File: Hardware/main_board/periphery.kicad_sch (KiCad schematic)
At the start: 67 parts, among them J4 SD, J5 NFC, J6 EXT1, J7 EXT0, U12 LP5562TMX

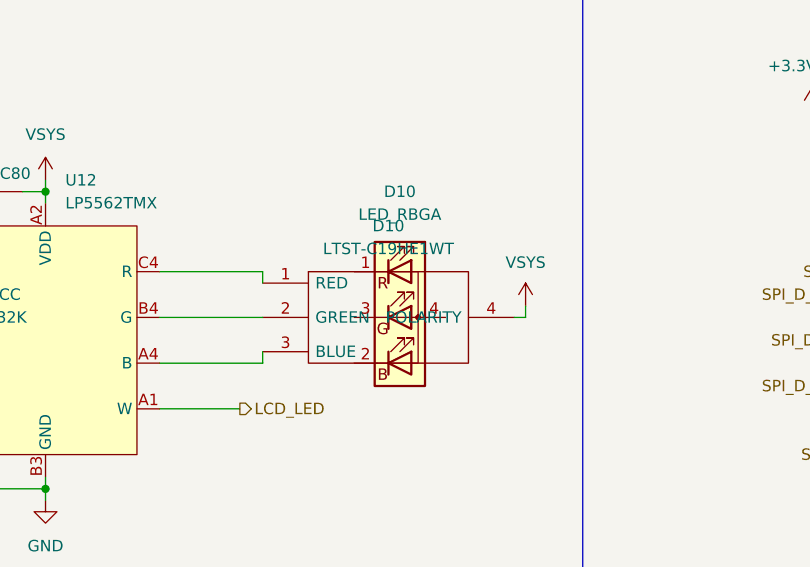
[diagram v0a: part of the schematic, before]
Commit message: misc: fix conflict
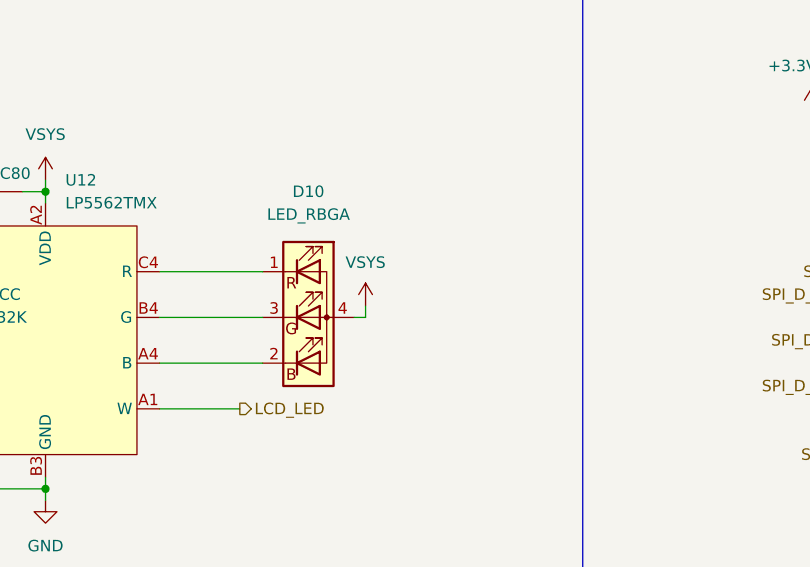
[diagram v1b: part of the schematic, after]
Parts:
- removed D10: LTST-C19HE1WT, Library:LTST-C19HE1WT, symbol Library:LTST-C19HE1WT
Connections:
- net VSYS: now also D10.4 (A)
- net at U12.C4 (R): now also D10.1 (RK)
- net at U12.B4 (G): now also D10.3 (GK)
- net at U12.A4 (B): now also D10.2 (BK)
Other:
- moved on the sheet: D10
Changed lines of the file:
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@@
 	(wire
 		(pts
-			(xy 74.93 44.45) (xy 74.93 45.72)
-		)
-		(stroke
-			(width 0)
-			(type default)
-		)
-	)
-	(wire
-		(pts
 			(xy 234.95 139.7) (xy 223.52 139.7)
 		)
@@
 	(wire
 		(pts
-			(xy 102.87 49.53) (xy 104.14 49.53)
+			(xy 85.09 49.53) (xy 86.36 49.53)
 		)
 		(stroke
@@
 	(wire
 		(pts
-			(xy 74.93 54.61) (xy 74.93 53.34)
-		)
-		(stroke
-			(width 0)
-			(type default)
-		)
-	)
-	(wire
-		(pts
 			(xy 78.74 144.78) (xy 85.09 144.78)
 		)
@@
 	(wire
 		(pts
-			(xy 104.14 49.53) (xy 104.14 48.26)
+			(xy 86.36 49.53) (xy 86.36 48.26)
 		)
 		(stroke
@@
 	)
 	(symbol
-		(lib_id "Library:LTST-C19HE1WT")
-		(at 74.93 45.72 0)
-		(unit 1)
-		(exclude_from_sim no)
-		(in_bom yes)
-		(on_board yes)
-		(dnp no)
-		(fields_autoplaced yes)
-		(property "Reference" "D10"
-			(at 88.9 39.37 0)
-			(effects
-				(font
-					(size 1.27 1.27)
-				)
-			)
-		)
-		(property "Value" "LTST-C19HE1WT"
-			(at 88.9 41.91 0)
-			(effects
-				(font
-					(size 1.27 1.27)
-				)
-			)
-		)
-		(property "Footprint" "Library:LTST-C19HE1WT"
-			(at 130.556 37.338 0)
-			(effects
-				(font
-					(size 1.27 1.27)
-				)
-				(justify left)
-				(hide yes)
-			)
-		)
-		(property "Datasheet" "https://datasheet.datasheetarchive.com/originals/distributors/Datasheets-DGA13/1159767.pdf"
-			(at 130.556 39.878 0)
-			(effects
-				(font
-					(size 1.27 1.27)
-				)
-				(justify left)
-				(hide yes)
-			)
-		)
-		(property "Description" "LED,SMD,1.6x1.5x0.4mm,Red/Green/Blue Lite-On LTST-C19HE1WT 3 RGB LED, 470 / 525 / 624 nm 3-Pin, Rectangle Lens SMD package"
-			(at 130.556 42.418 0)
-			(effects
-				(font
-					(size 1.27 1.27)
-				)
-				(justify left)
-				(hide yes)
-			)
-		)
-		(property "Height" ""
-			(at 106.68 50.8 0)
-			(effects
-				(font
-					(size 1.27 1.27)
-				)
-				(justify left)
-				(hide yes)
-			)
-		)
-		(property "Mouser Part Number" "859-LTST-C19HE1WT"
-			(at 130.556 47.498 0)
-			(effects
-				(font
-					(size 1.27 1.27)
-				)
-				(justify left)
-				(hide yes)
-			)
-		)
-		(property "Mouser Price/Stock" "https://www.mouser.co.uk/ProductDetail/Lite-On/LTST-C19HE1WT?qs=WAWaI72GHKxJLPArJA9%252BUw%3D%3D"
-			(at 130.556 50.038 0)
-			(effects
-				(font
-					(size 1.27 1.27)
-				)
-				(justify left)
-				(hide yes)
-			)
-		)
-		(property "Manufacturer_Name" "Lite-On"
-			(at 130.556 52.578 0)
-			(effects
-				(font
-					(size 1.27 1.27)
-				)
-				(justify left)
-				(hide yes)
-			)
-		)
-		(property "Manufacturer_Part_Number" "LTST-C19HE1WT"
-			(at 130.556 55.118 0)
-			(effects
-				(font
-					(size 1.27 1.27)
-				)
-				(justify left)
-				(hide yes)
-			)
-		)
-		(pin "3"
-		)
-		(pin "4"
-		)
-		(pin "2"
-		)
-		(pin "1"
-		)
-		(instances
-			(project "main_board"
-				(path "/16216a68-6dea-41d7-8e15-2cc84f72f8e2/07054158-43be-4dab-a684-c4a4bca9b970"
-					(reference "D10")
-					(unit 1)
-				)
-			)
-		)
-	)
-	(symbol
 		(lib_id "Device:R_US")
 		(at 147.32 35.56 180)
@@
 	(symbol
 		(lib_id "Device:LED_RBGA")
-		(at 90.17 49.53 0)
+		(at 80.01 49.53 0)
 		(unit 1)
 		(exclude_from_sim no)
@@
 		(fields_autoplaced yes)
 		(property "Reference" "D10"
-			(at 90.17 35.56 0)
+			(at 80.01 35.56 0)
 			(effects
 				(font
@@
 		)
 		(property "Value" "LED_RBGA"
-			(at 90.17 38.1 0)
+			(at 80.01 38.1 0)
 			(effects
 				(font
@@
 		)
 		(property "Footprint" "Library:LTST-C19HE1WT_LTO"
-			(at 90.17 50.8 0)
+			(at 80.01 50.8 0)
 			(effects
 				(font
@@
 		)
 		(property "Datasheet" "~"
-			(at 90.17 50.8 0)
+			(at 80.01 50.8 0)
 			(effects
 				(font
@@
 		)
 		(property "Description" "RGB LED, red/blue/green/anode"
-			(at 90.17 49.53 0)
+			(at 80.01 49.53 0)
 			(effects
 				(font
@@
 	(symbol
 		(lib_id "power:+3.3V")
-		(at 104.14 48.26 0)
+		(at 86.36 48.26 0)
 		(unit 1)
 		(exclude_from_sim no)
@@
 		(dnp no)
 		(property "Reference" "#PWR0122"
-			(at 104.14 52.07 0)
+			(at 86.36 52.07 0)
 			(effects
 				(font
@@
 		)
 		(property "Value" "VSYS"
-			(at 104.14 43.434 0)
+			(at 86.36 43.434 0)
 			(effects
 				(font
@@
 		)
 		(property "Footprint" ""
-			(at 104.14 48.26 0)
+			(at 86.36 48.26 0)
 			(effects
 				(font
@@
 		)
 		(property "Datasheet" ""
-			(at 104.14 48.26 0)
+			(at 86.36 48.26 0)
 			(effects
 				(font
@@
 		)
 		(property "Description" "Power symbol creates a global label with name \"+3.3V\""
-			(at 104.14 48.26 0)
+			(at 86.36 48.26 0)
 			(effects
 				(font

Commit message: footprint: change sd card footprint
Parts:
- J4: footprint Library:TF-SMD_TF-110 -> Library:CONN_503398-1892_MOL
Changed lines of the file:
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@@
 			)
 		)
-		(property "Footprint" "Library:TF-SMD_TF-110"
+		(property "Footprint" "Library:CONN_503398-1892_MOL"
 			(at 292.1 34.29 0)
 			(effects
